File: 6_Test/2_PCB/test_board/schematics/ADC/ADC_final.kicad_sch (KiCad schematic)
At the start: 19 parts, among them J1 BNC1, J2 BNC2, J3 TSW-107-07-F-D, J4 TSW-107-07-F-D

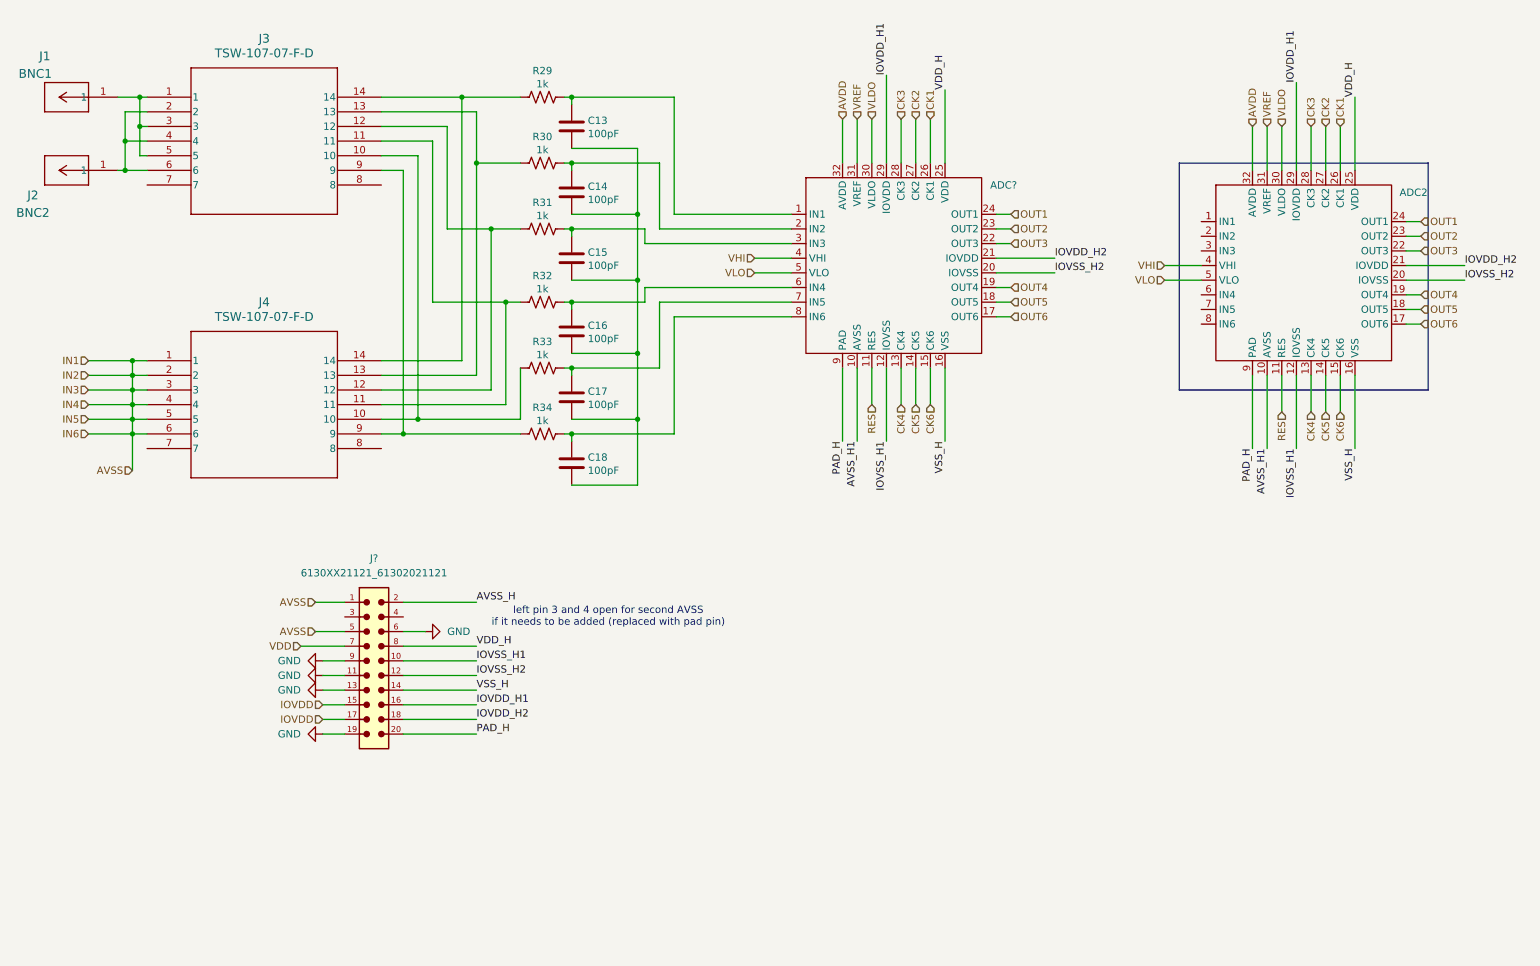
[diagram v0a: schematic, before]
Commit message: Corrections to schematic 11_20_24
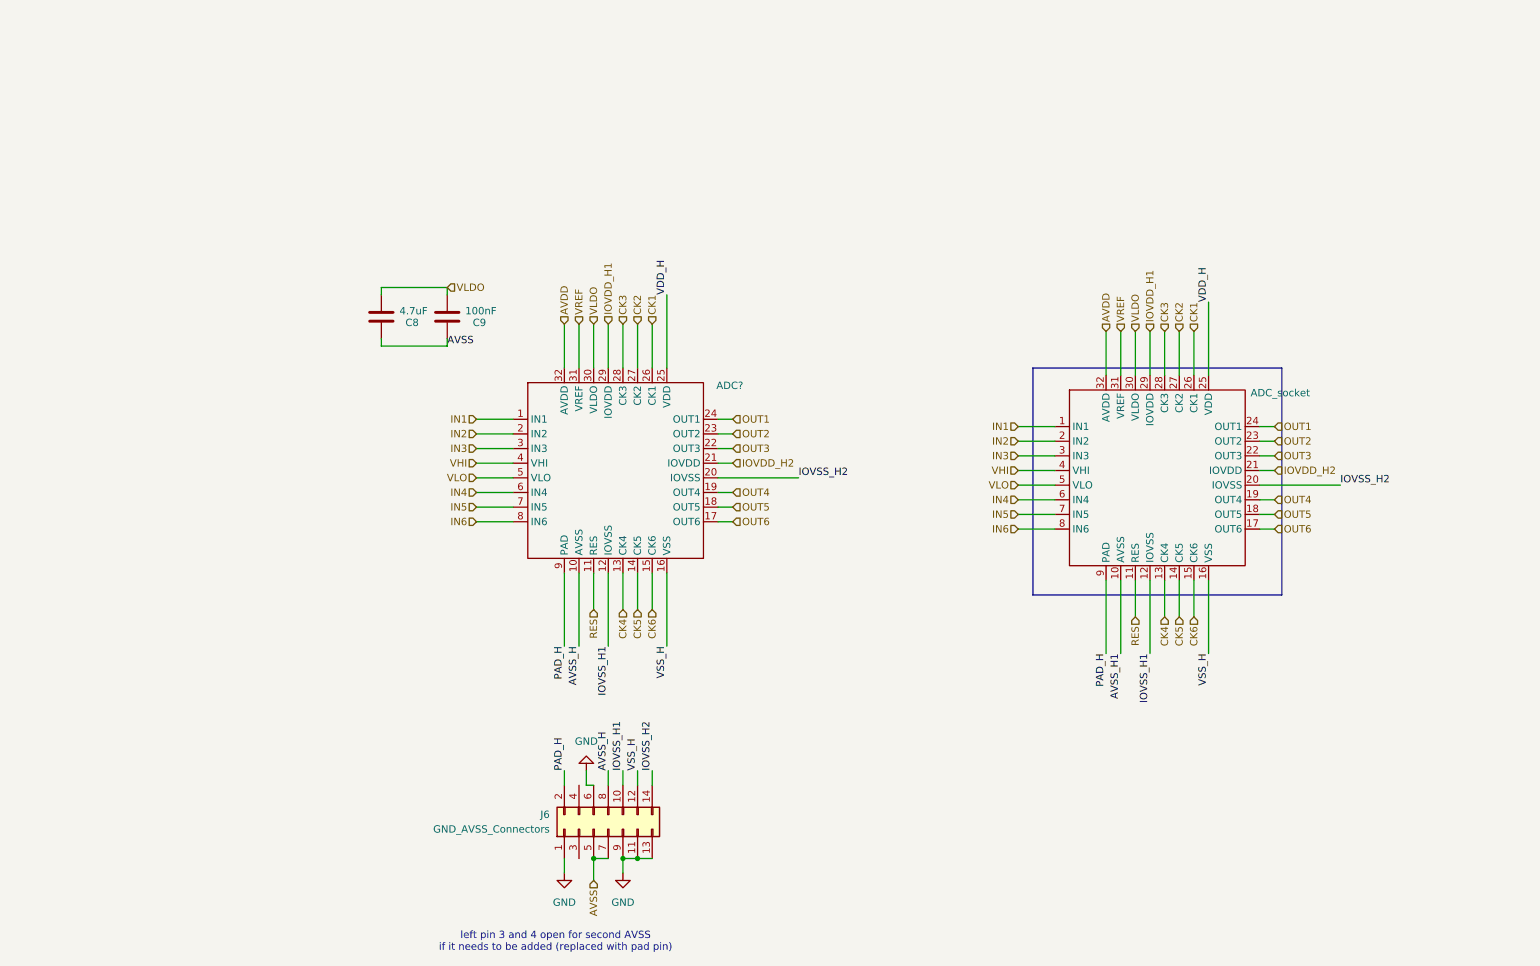
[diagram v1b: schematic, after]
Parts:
- removed C13, C14, C15, C16, C17, C18: 100pF, symbol Device:C
- removed J1: BNC1, CONN_1274571-1_TYCO, symbol bnc_mini:1274571-1
- removed J2: BNC2, CONN_1274571-1_TYCO, symbol bnc_mini:1274571-1
- removed J3, J4: TSW-107-07-F-D, TSW-107-07-G-D_SAI, symbol 6x2Header:TSW-107-07-F-D
- removed J?: 6130XX21121_61302021121, 6130XX21121_61302021121:61302021121, symbol 2x10Header:6130XX21121_61302021121
- removed R29, R30, R31, R32, R33, R34: 1k, symbol Device:R_US
- added C8: 4.7uF, Capacitor_SMD:C_0201_0603Metric, symbol Device:C
- added C9: 100nF, Capacitor_SMD:C_0201_0603Metric, symbol Device:C
- added J6: GND_AVSS_Connectors, Connector_PinHeader_2.54mm:PinHeader_2x07_P2.54mm_Vertical, symbol Connector_Generic:Conn_02x07_Odd_Even
- renumbered ADC2 to ADC_socket
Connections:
- net AVSS: now also C8.2, C9.2, J6.5 (Pin_5), J6.7 (Pin_7)
- net AVSS_H: now also ADC?.10 (AVSS), J6.8 (Pin_8)
- net AVSS_H1: no longer ADC?.10 (AVSS)
- net GND: now also J6.1 (Pin_1), J6.11 (Pin_11), J6.13 (Pin_13), J6.6 (Pin_6), J6.9 (Pin_9)
- net IOVSS_H1: now also J6.10 (Pin_10)
- net IOVSS_H2: now also J6.14 (Pin_14)
- net PAD_H: now also J6.2 (Pin_2)
- net VLDO: now also C8.1, C9.1
- net VSS_H: now also J6.12 (Pin_12)
- net IN5: now reaches ADC?.7 (IN5)
- net IN5: now also ADC_socket.7 (IN5)
- net IN2: now reaches ADC?.2 (IN2)
- net IN2: now also ADC_socket.2 (IN2)
- net IN4: now reaches ADC?.6 (IN4)
- net IN4: now also ADC_socket.6 (IN4)
- net IN6: now reaches ADC?.8 (IN6)
- net IN6: now also ADC_socket.8 (IN6)
- net IN1: now reaches ADC?.1 (IN1)
- net IN1: now also ADC_socket.1 (IN1)
- net IN3: now reaches ADC?.3 (IN3)
- net IN3: now also ADC_socket.3 (IN3)
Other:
- moved on the sheet: ADC?, ADC_socket
